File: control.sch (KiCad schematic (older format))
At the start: 37 parts, among them K1 G5Q-1A, K2 G5Q-1A, K3 RT42xxxx, K4 RT42xxxx, K5 FINDER-32.21-x300, K6 FINDER-32.21-x300, T1 Transformer_TEZ_22x24_6V, U1 LTV-817, U2 ULN2003A, U3 LTV-817, U4 MOC3060S, U5 MOC3060S

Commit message: tarpinis komitas
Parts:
- removed D2: LL4148, Diode_SMD:D_MiniMELF, symbol Diode:LL4148
- removed D3, D4: Z0103MN, Package_TO_SOT_SMD:SOT-223, symbol Triac_Thyristor:Z0103MN
- removed F1: 3A, Fuse:Fuseholder_Cylinder-5x20mm_Schurter_0031_8201_Horizontal_Open, symbol Device:Fuse
- removed K1, K2: G5Q-1A, Relay_THT:Relay_SPDT_Finder_34.51_Vertical, symbol Relay:G5Q-1A
- removed K3, K4: RT42xxxx, Relay_THT:Relay_DPDT_Schrack-RT2-FormC_RM5mm, symbol Relay:RT42xxxx
- removed K5, K6: FINDER-32.21-x300, Relay_THT:Relay_SPST_Schrack-RT1-FormA_RM5mm, symbol Relay:FINDER-32.21-x300
- removed R10, R11, R13, R14: 33k, Resistor_SMD:R_1206_3216Metric_Pad1.42x1.75mm_HandSolder, symbol Device:R
- removed R12, R15, R16, R17, R18, R9: R, Resistor_SMD:R_0805_2012Metric_Pad1.15x1.40mm_HandSolder, symbol Device:R
- removed U3: LTV-817, Package_DIP:DIP-4_W7.62mm, symbol Isolator:LTV-817
- removed U4, U5: MOC3060S, disc:DIP-6_W9.53mm_SMD, symbol disc:MOC3060S
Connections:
- net labels removed: ACL, ACN, AirExtractor_L, AirExtractor_N, EAKITCHN, EAWCN, EHALLLIGHT, EHALLLIGHT_N, ExtractAir_KITCH, ExtractAir_WC, ISOCKN, LIGHTBASH1, LIGHTBASH2, LIGHTON, LIGHTWC1, LIGHTWC2, WORKLIGHT, WORKLIGHT_N, iSocket
- wire segments 165 -> 53
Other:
- note removed: "Arkos rozete"
- note removed: "Garu surinktuvas"
- note removed: "Koridoriaus\napsvietimas"
- note removed: "Virtuves darbo\nzonos apsvietimas"
- note removed: "Virtuves\nventiliatorius"
- note removed: "Vonios apsvietimas\n230VAC"
- note removed: "Vonios ir WC\nventiliatorius"
- note removed: "WC apsvietimas\n230VAC"

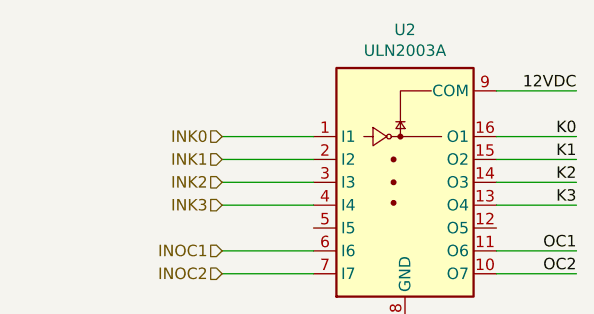
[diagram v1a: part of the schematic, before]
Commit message: schemos paruosimas
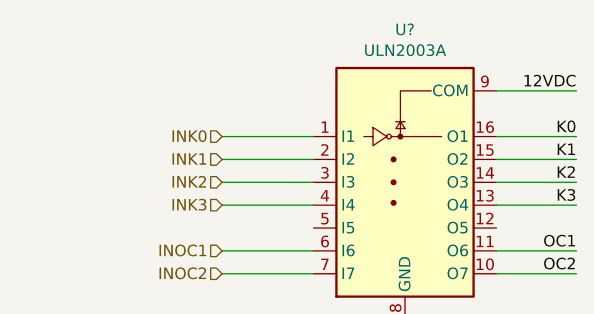
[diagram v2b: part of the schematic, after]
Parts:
- renumbered C1 to C?, D1 to D?, R5 to R?, R7 to R?, R4 to R?, R3 to R?, R2 to R?, R1 to R?, R6 to R?, R8 to R?, T1 to T?, TH1 to TH?, U2 to U?, U1 to U?
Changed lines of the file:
@@
 $EndDescr
 $Comp
-L Transistor_Array:ULN2003A U2
+L Transistor_Array:ULN2003A U?
 U 1 1 5BC77E03
 P 13450 2150
-F 0 "U2" H 13450 2817 50  0000 C CNN
+F 0 "U?" H 13450 2817 50  0000 C CNN
 F 1 "ULN2003A" H 13450 2726 50  0000 C CNN
 F 2 "" H 13500 1600 50  0001 L CNN
@@
 OC1
 $Comp
-L Isolator:LTV-817 U1
+L Isolator:LTV-817 U?
 U 1 1 5BC77E06
 P 2650 8900
-F 0 "U1" H 2650 9225 50  0000 C CNN
+F 0 "U?" H 2650 9225 50  0000 C CNN
 F 1 "LTV-817" H 2650 9134 50  0000 C CNN
 F 2 "Package_DIP:DIP-4_W7.62mm" H 2450 8700 50  0001 L CIN
@@
 COM
 $Comp
-L Diode:LL4148 D1
+L Diode:LL4148 D?
 U 1 1 5BC77E07
 P 3250 8900
-F 0 "D1" V 3204 8979 50  0000 L CNN
+F 0 "D?" V 3204 8979 50  0000 L CNN
 F 1 "LL4148" V 3295 8979 50  0000 L CNN
 F 2 "Diode_SMD:D_MiniMELF" H 3250 8725 50  0001 C CNN
@@
 Connection ~ 3250 9150
 $Comp
-L Device:R R5
+L Device:R R?
 U 1 1 5BC77E08
 P 3650 8650
-F 0 "R5" V 3550 8550 50  0000 C CNN
+F 0 "R?" V 3550 8550 50  0000 C CNN
 F 1 "33k" V 3550 8750 50  0000 C CNN
 F 2 "Resistor_SMD:R_1206_3216Metric_Pad1.42x1.75mm_HandSolder" V 3580 8650 50  0001 C CNN
@@
 $EndComp
 $Comp
-L Device:R R6
+L Device:R R?
 U 1 1 5BC8FFB1
 P 3650 9150
-F 0 "R6" V 3550 9050 50  0000 C CNN
+F 0 "R?" V 3550 9050 50  0000 C CNN
 F 1 "33k" V 3550 9250 50  0000 C CNN
 F 2 "Resistor_SMD:R_1206_3216Metric_Pad1.42x1.75mm_HandSolder" V 3580 9150 50  0001 C CNN
@@
 $EndComp
 $Comp
-L Device:R R7
+L Device:R R?
 U 1 1 5BC77E0A
 P 4050 8650
-F 0 "R7" V 3950 8550 50  0000 C CNN
+F 0 "R?" V 3950 8550 50  0000 C CNN
 F 1 "33k" V 3950 8750 50  0000 C CNN
 F 2 "Resistor_SMD:R_1206_3216Metric_Pad1.42x1.75mm_HandSolder" V 3980 8650 50  0001 C CNN
@@
 $EndComp
 $Comp
-L Device:R R8
+L Device:R R?
 U 1 1 5BC90060
 P 4050 9150
-F 0 "R8" V 3950 9050 50  0000 C CNN
+F 0 "R?" V 3950 9050 50  0000 C CNN
 F 1 "33k" V 3950 9250 50  0000 C CNN
 F 2 "Resistor_SMD:R_1206_3216Metric_Pad1.42x1.75mm_HandSolder" V 3980 9150 50  0001 C CNN
@@
 VREF
 $Comp
-L capacitors:CP_100uFx16V C1
+L capacitors:CP_100uFx16V C?
 U 1 1 5BC1DECF
 P 3000 10100
-F 0 "C1" H 2700 10150 50  0000 L CNN
+F 0 "C?" H 2700 10150 50  0000 L CNN
 F 1 "100uFx16V" H 2450 10050 50  0000 L CNN
 F 2 "Capacitors_SMD:CP_Elec_6.3x5.7" H 3850 10350 50  0001 C CNN
@@
 230N
 $Comp
-L disc:Transformer_TEZ_22x24_6V T1
+L disc:Transformer_TEZ_22x24_6V T?
 U 1 1 5BCA7928
 P 3900 9700
-F 0 "T1" H 3900 9987 50  0000 C CNN
+F 0 "T?" H 3900 9987 50  0000 C CNN
 F 1 "Transformer_TEZ_22x24_6V" H 3900 9987 50  0001 C CNN
 F 2 "Transformer_THT:Transformer_Breve_TEZ-22x24" H 5300 9800 50  0001 C CNN
@@
 	4500 9500 4600 9500
 $Comp
-L Device:Thermistor_PTC TH1
+L Device:Thermistor_PTC TH?
 U 1 1 5BC77E0F
 P 4750 9500
-F 0 "TH1" V 4600 9450 50  0000 C CNN
+F 0 "TH?" V 4600 9450 50  0000 C CNN
 F 1 "230V/150mA" V 4900 9500 50  0000 C CNN
 F 2 "" H 4800 9300 50  0001 L CNN
@@
 INOC2
 $Comp
-L Device:R R4
+L Device:R R?
 U 1 1 5BC77E14
 P 3250 9500
-F 0 "R4" V 3150 9400 50  0000 C CNN
+F 0 "R?" V 3150 9400 50  0000 C CNN
 F 1 "1k" V 3150 9600 50  0000 C CNN
 F 2 "Resistor_SMD:R_0805_2012Metric_Pad1.15x1.40mm_HandSolder" V 3180 9500 50  0001 C CNN
@@
 $EndComp
 $Comp
-L Device:R R3
+L Device:R R?
 U 1 1 5BC77E15
 P 3000 9700
-F 0 "R3" H 3150 9750 50  0000 C CNN
+F 0 "R?" H 3150 9750 50  0000 C CNN
 F 1 "120" H 3150 9650 50  0000 C CNN
 F 2 "Resistor_SMD:R_0805_2012Metric_Pad1.15x1.40mm_HandSolder" V 2930 9700 50  0001 C CNN
@@
 $EndComp
 $Comp
-L Device:R R2
+L Device:R R?
 U 1 1 5BC77E16
 P 2500 10100
-F 0 "R2" H 2650 10150 50  0000 C CNN
+F 0 "R?" H 2650 10150 50  0000 C CNN
 F 1 "Rx" H 2650 10050 50  0000 C CNN
 F 2 "Resistor_SMD:R_0805_2012Metric_Pad1.15x1.40mm_HandSolder" V 2430 10100 50  0001 C CNN
@@
 $EndComp
 $Comp
-L Device:R R1
+L Device:R R?
 U 1 1 5BC77E17
 P 2250 9900
-F 0 "R1" V 2350 10000 50  0000 C CNN
+F 0 "R?" V 2350 10000 50  0000 C CNN
 F 1 "Rx" V 2350 9850 50  0000 C CNN
 F 2 "Resistor_SMD:R_0805_2012Metric_Pad1.15x1.40mm_HandSolder" V 2180 9900 50  0001 C CNN

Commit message: tarpinis kommitas
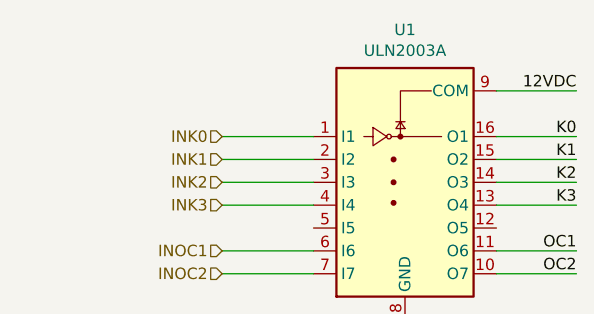
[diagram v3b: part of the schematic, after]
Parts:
- gave numbers to parts that had none: 14
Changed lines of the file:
@@
 $Descr A3 16535 11693
 encoding utf-8
-Sheet 2 3
+Sheet 2 4
 Title ""
 Date ""
@@
 $EndDescr
 $Comp
-L Transistor_Array:ULN2003A U?
+L Transistor_Array:ULN2003A U1
 U 1 1 5BC77E03
 P 13450 2150
-F 0 "U?" H 13450 2817 50  0000 C CNN
+F 0 "U1" H 13450 2817 50  0000 C CNN
 F 1 "ULN2003A" H 13450 2726 50  0000 C CNN
 F 2 "" H 13500 1600 50  0001 L CNN
@@
 OC1
 $Comp
-L Isolator:LTV-817 U?
+L Isolator:LTV-817 U2
 U 1 1 5BC77E06
 P 2650 8900
-F 0 "U?" H 2650 9225 50  0000 C CNN
+F 0 "U2" H 2650 9225 50  0000 C CNN
 F 1 "LTV-817" H 2650 9134 50  0000 C CNN
 F 2 "Package_DIP:DIP-4_W7.62mm" H 2450 8700 50  0001 L CIN
@@
 COM
 $Comp
-L Diode:LL4148 D?
+L Diode:LL4148 D1
 U 1 1 5BC77E07
 P 3250 8900
-F 0 "D?" V 3204 8979 50  0000 L CNN
+F 0 "D1" V 3204 8979 50  0000 L CNN
 F 1 "LL4148" V 3295 8979 50  0000 L CNN
 F 2 "Diode_SMD:D_MiniMELF" H 3250 8725 50  0001 C CNN
@@
 Connection ~ 3250 9150
 $Comp
-L Device:R R?
+L Device:R R1
 U 1 1 5BC77E08
 P 3650 8650
-F 0 "R?" V 3550 8550 50  0000 C CNN
+F 0 "R1" V 3550 8550 50  0000 C CNN
 F 1 "33k" V 3550 8750 50  0000 C CNN
 F 2 "Resistor_SMD:R_1206_3216Metric_Pad1.42x1.75mm_HandSolder" V 3580 8650 50  0001 C CNN
@@
 $EndComp
 $Comp
-L Device:R R?
+L Device:R R3
 U 1 1 5BC8FFB1
 P 3650 9150
-F 0 "R?" V 3550 9050 50  0000 C CNN
+F 0 "R3" V 3550 9050 50  0000 C CNN
 F 1 "33k" V 3550 9250 50  0000 C CNN
 F 2 "Resistor_SMD:R_1206_3216Metric_Pad1.42x1.75mm_HandSolder" V 3580 9150 50  0001 C CNN
@@
 $EndComp
 $Comp
-L Device:R R?
+L Device:R R2
 U 1 1 5BC77E0A
 P 4050 8650
-F 0 "R?" V 3950 8550 50  0000 C CNN
+F 0 "R2" V 3950 8550 50  0000 C CNN
 F 1 "33k" V 3950 8750 50  0000 C CNN
 F 2 "Resistor_SMD:R_1206_3216Metric_Pad1.42x1.75mm_HandSolder" V 3980 8650 50  0001 C CNN
@@
 $EndComp
 $Comp
-L Device:R R?
+L Device:R R4
 U 1 1 5BC90060
 P 4050 9150
-F 0 "R?" V 3950 9050 50  0000 C CNN
+F 0 "R4" V 3950 9050 50  0000 C CNN
 F 1 "33k" V 3950 9250 50  0000 C CNN
 F 2 "Resistor_SMD:R_1206_3216Metric_Pad1.42x1.75mm_HandSolder" V 3980 9150 50  0001 C CNN
@@
 VREF
 $Comp
-L capacitors:CP_100uFx16V C?
+L capacitors:CP_100uFx16V C1
 U 1 1 5BC1DECF
 P 3000 10100
-F 0 "C?" H 2700 10150 50  0000 L CNN
+F 0 "C1" H 2700 10150 50  0000 L CNN
 F 1 "100uFx16V" H 2450 10050 50  0000 L CNN
 F 2 "Capacitors_SMD:CP_Elec_6.3x5.7" H 3850 10350 50  0001 C CNN
@@
 230N
 $Comp
-L disc:Transformer_TEZ_22x24_6V T?
+L disc:Transformer_TEZ_22x24_6V T1
 U 1 1 5BCA7928
 P 3900 9700
-F 0 "T?" H 3900 9987 50  0000 C CNN
+F 0 "T1" H 3900 9987 50  0000 C CNN
 F 1 "Transformer_TEZ_22x24_6V" H 3900 9987 50  0001 C CNN
 F 2 "Transformer_THT:Transformer_Breve_TEZ-22x24" H 5300 9800 50  0001 C CNN
@@
 	4500 9500 4600 9500
 $Comp
-L Device:Thermistor_PTC TH?
+L Device:Thermistor_PTC TH1
 U 1 1 5BC77E0F
 P 4750 9500
-F 0 "TH?" V 4600 9450 50  0000 C CNN
+F 0 "TH1" V 4600 9450 50  0000 C CNN
 F 1 "230V/150mA" V 4900 9500 50  0000 C CNN
 F 2 "" H 4800 9300 50  0001 L CNN
@@
 INOC2
 $Comp
-L Device:R R?
+L Device:R R5
 U 1 1 5BC77E14
 P 3250 9500
-F 0 "R?" V 3150 9400 50  0000 C CNN
+F 0 "R5" V 3150 9400 50  0000 C CNN
 F 1 "1k" V 3150 9600 50  0000 C CNN
 F 2 "Resistor_SMD:R_0805_2012Metric_Pad1.15x1.40mm_HandSolder" V 3180 9500 50  0001 C CNN
@@
 $EndComp
 $Comp
-L Device:R R?
+L Device:R R6
 U 1 1 5BC77E15
 P 3000 9700
-F 0 "R?" H 3150 9750 50  0000 C CNN
+F 0 "R6" H 3150 9750 50  0000 C CNN
 F 1 "120" H 3150 9650 50  0000 C CNN
 F 2 "Resistor_SMD:R_0805_2012Metric_Pad1.15x1.40mm_HandSolder" V 2930 9700 50  0001 C CNN
@@
 $EndComp
 $Comp
-L Device:R R?
+L Device:R R8
 U 1 1 5BC77E16
 P 2500 10100
-F 0 "R?" H 2650 10150 50  0000 C CNN
+F 0 "R8" H 2650 10150 50  0000 C CNN
 F 1 "Rx" H 2650 10050 50  0000 C CNN
 F 2 "Resistor_SMD:R_0805_2012Metric_Pad1.15x1.40mm_HandSolder" V 2430 10100 50  0001 C CNN
@@
 $EndComp
 $Comp
-L Device:R R?
+L Device:R R7
 U 1 1 5BC77E17
 P 2250 9900
-F 0 "R?" V 2350 10000 50  0000 C CNN
+F 0 "R7" V 2350 10000 50  0000 C CNN
 F 1 "Rx" V 2350 9850 50  0000 C CNN
 F 2 "Resistor_SMD:R_0805_2012Metric_Pad1.15x1.40mm_HandSolder" V 2180 9900 50  0001 C CNN

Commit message: tarpinis kommitas
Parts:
- C1: symbol capacitors:CP_100uFx16V -> ihouse-rescue:capacitors_CP_100uFx16V-ihouse-rescue
- D1: symbol Diode:LL4148 -> ihouse-rescue:Diode_LL4148-ihouse-rescue
- R1: renamed from R7; symbol Device:R -> ihouse-rescue:Device_R-ihouse-rescue
- R2: renamed from R8; symbol Device:R -> ihouse-rescue:Device_R-ihouse-rescue
- R3: renamed from R6; symbol Device:R -> ihouse-rescue:Device_R-ihouse-rescue
- R4: renamed from R5; symbol Device:R -> ihouse-rescue:Device_R-ihouse-rescue
- R5: renamed from R1; symbol Device:R -> ihouse-rescue:Device_R-ihouse-rescue
- R6: renamed from R3; symbol Device:R -> ihouse-rescue:Device_R-ihouse-rescue
- R7: renamed from R2; symbol Device:R -> ihouse-rescue:Device_R-ihouse-rescue
- R8: renamed from R4; symbol Device:R -> ihouse-rescue:Device_R-ihouse-rescue
- T1: symbol disc:Transformer_TEZ_22x24_6V -> ihouse-rescue:disc_Transformer_TEZ_22x24_6V-ihouse-rescue
- TH1: symbol Device:Thermistor_PTC -> ihouse-rescue:Device_Thermistor_PTC-ihouse-rescue
- U1: renamed from U2; symbol Isolator:LTV-817 -> ihouse-rescue:Isolator_LTV-817-ihouse-rescue
- U2: renamed from U1; symbol Transistor_Array:ULN2003A -> ihouse-rescue:Transistor_Array_ULN2003A-ihouse-rescue
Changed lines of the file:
@@
 $EndDescr
 $Comp
-L Transistor_Array:ULN2003A U1
+L ihouse-rescue:Transistor_Array_ULN2003A-ihouse-rescue U2
 U 1 1 5BC77E03
 P 13450 2150
-F 0 "U1" H 13450 2817 50  0000 C CNN
+F 0 "U2" H 13450 2817 50  0000 C CNN
 F 1 "ULN2003A" H 13450 2726 50  0000 C CNN
 F 2 "" H 13500 1600 50  0001 L CNN
@@
 OC1
 $Comp
-L Isolator:LTV-817 U2
+L ihouse-rescue:Isolator_LTV-817-ihouse-rescue U1
 U 1 1 5BC77E06
 P 2650 8900
-F 0 "U2" H 2650 9225 50  0000 C CNN
+F 0 "U1" H 2650 9225 50  0000 C CNN
 F 1 "LTV-817" H 2650 9134 50  0000 C CNN
 F 2 "Package_DIP:DIP-4_W7.62mm" H 2450 8700 50  0001 L CIN
@@
 COM
 $Comp
-L Diode:LL4148 D1
+L ihouse-rescue:Diode_LL4148-ihouse-rescue D1
 U 1 1 5BC77E07
 P 3250 8900
@@
 Connection ~ 3250 9150
 $Comp
-L Device:R R1
+L ihouse-rescue:Device_R-ihouse-rescue R5
 U 1 1 5BC77E08
 P 3650 8650
-F 0 "R1" V 3550 8550 50  0000 C CNN
+F 0 "R5" V 3550 8550 50  0000 C CNN
 F 1 "33k" V 3550 8750 50  0000 C CNN
 F 2 "Resistor_SMD:R_1206_3216Metric_Pad1.42x1.75mm_HandSolder" V 3580 8650 50  0001 C CNN
@@
 $EndComp
 $Comp
-L Device:R R3
+L ihouse-rescue:Device_R-ihouse-rescue R6
 U 1 1 5BC8FFB1
 P 3650 9150
-F 0 "R3" V 3550 9050 50  0000 C CNN
+F 0 "R6" V 3550 9050 50  0000 C CNN
 F 1 "33k" V 3550 9250 50  0000 C CNN
 F 2 "Resistor_SMD:R_1206_3216Metric_Pad1.42x1.75mm_HandSolder" V 3580 9150 50  0001 C CNN
@@
 $EndComp
 $Comp
-L Device:R R2
+L ihouse-rescue:Device_R-ihouse-rescue R7
 U 1 1 5BC77E0A
 P 4050 8650
-F 0 "R2" V 3950 8550 50  0000 C CNN
+F 0 "R7" V 3950 8550 50  0000 C CNN
 F 1 "33k" V 3950 8750 50  0000 C CNN
 F 2 "Resistor_SMD:R_1206_3216Metric_Pad1.42x1.75mm_HandSolder" V 3980 8650 50  0001 C CNN
@@
 $EndComp
 $Comp
-L Device:R R4
+L ihouse-rescue:Device_R-ihouse-rescue R8
 U 1 1 5BC90060
 P 4050 9150
-F 0 "R4" V 3950 9050 50  0000 C CNN
+F 0 "R8" V 3950 9050 50  0000 C CNN
 F 1 "33k" V 3950 9250 50  0000 C CNN
 F 2 "Resistor_SMD:R_1206_3216Metric_Pad1.42x1.75mm_HandSolder" V 3980 9150 50  0001 C CNN
@@
 VREF
 $Comp
-L capacitors:CP_100uFx16V C1
+L ihouse-rescue:capacitors_CP_100uFx16V-ihouse-rescue C1
 U 1 1 5BC1DECF
 P 3000 10100
@@
 230N
 $Comp
-L disc:Transformer_TEZ_22x24_6V T1
+L ihouse-rescue:disc_Transformer_TEZ_22x24_6V-ihouse-rescue T1
 U 1 1 5BCA7928
 P 3900 9700
@@
 	4500 9500 4600 9500
 $Comp
-L Device:Thermistor_PTC TH1
+L ihouse-rescue:Device_Thermistor_PTC-ihouse-rescue TH1
 U 1 1 5BC77E0F
 P 4750 9500
@@
 INOC2
 $Comp
-L Device:R R5
+L ihouse-rescue:Device_R-ihouse-rescue R4
 U 1 1 5BC77E14
 P 3250 9500
-F 0 "R5" V 3150 9400 50  0000 C CNN
+F 0 "R4" V 3150 9400 50  0000 C CNN
 F 1 "1k" V 3150 9600 50  0000 C CNN
 F 2 "Resistor_SMD:R_0805_2012Metric_Pad1.15x1.40mm_HandSolder" V 3180 9500 50  0001 C CNN
@@
 $EndComp
 $Comp
-L Device:R R6
+L ihouse-rescue:Device_R-ihouse-rescue R3
 U 1 1 5BC77E15
 P 3000 9700
-F 0 "R6" H 3150 9750 50  0000 C CNN
+F 0 "R3" H 3150 9750 50  0000 C CNN
 F 1 "120" H 3150 9650 50  0000 C CNN
 F 2 "Resistor_SMD:R_0805_2012Metric_Pad1.15x1.40mm_HandSolder" V 2930 9700 50  0001 C CNN
@@
 $EndComp
 $Comp
-L Device:R R8
+L ihouse-rescue:Device_R-ihouse-rescue R2
 U 1 1 5BC77E16
 P 2500 10100
-F 0 "R8" H 2650 10150 50  0000 C CNN
+F 0 "R2" H 2650 10150 50  0000 C CNN
 F 1 "Rx" H 2650 10050 50  0000 C CNN
 F 2 "Resistor_SMD:R_0805_2012Metric_Pad1.15x1.40mm_HandSolder" V 2430 10100 50  0001 C CNN
@@
 $EndComp
 $Comp
-L Device:R R7
+L ihouse-rescue:Device_R-ihouse-rescue R1
 U 1 1 5BC77E17
 P 2250 9900
-F 0 "R7" V 2350 10000 50  0000 C CNN
+F 0 "R1" V 2350 10000 50  0000 C CNN
 F 1 "Rx" V 2350 9850 50  0000 C CNN
 F 2 "Resistor_SMD:R_0805_2012Metric_Pad1.15x1.40mm_HandSolder" V 2180 9900 50  0001 C CNN
